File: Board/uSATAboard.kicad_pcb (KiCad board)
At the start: 2 copper layers, 34.5 x 8.4 mm, 8 parts, among them CN2 USATA, P1 CONN_1, P2 CONN_1, P3 CONN_1, P4 CONN_1, P5 CONN_1, P6 CONN_1, P7 CONN_1

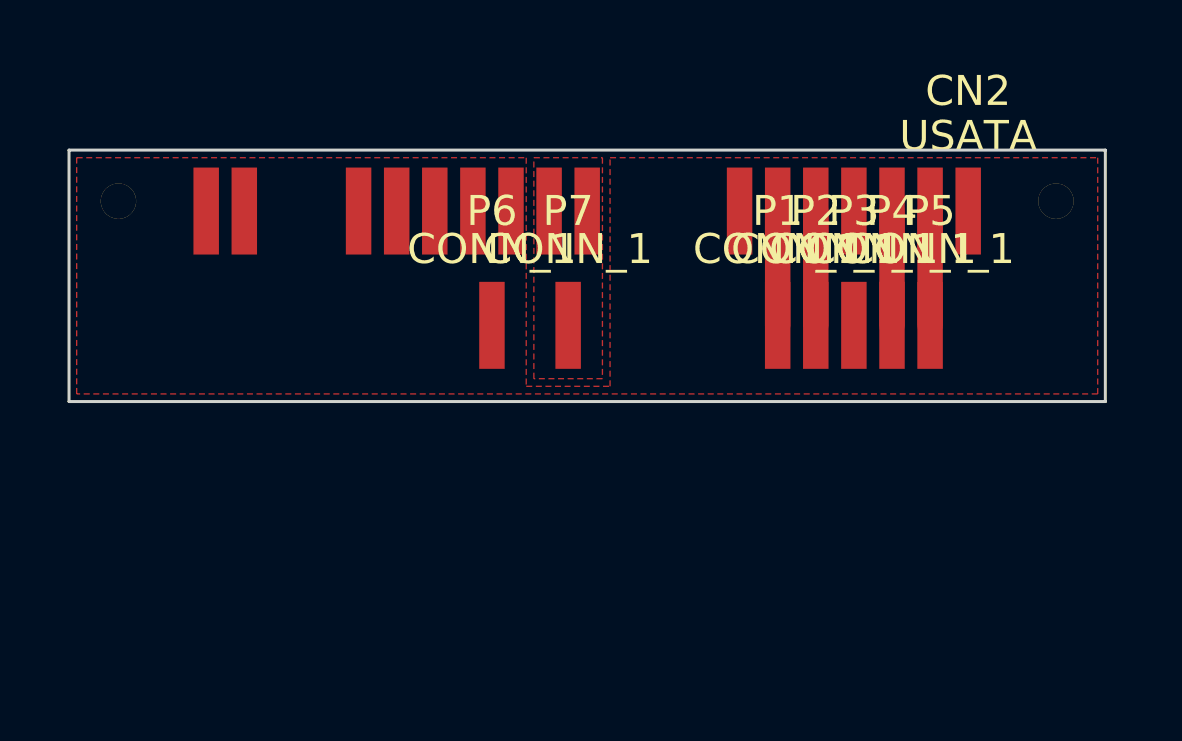
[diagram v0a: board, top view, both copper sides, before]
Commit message: final
for now
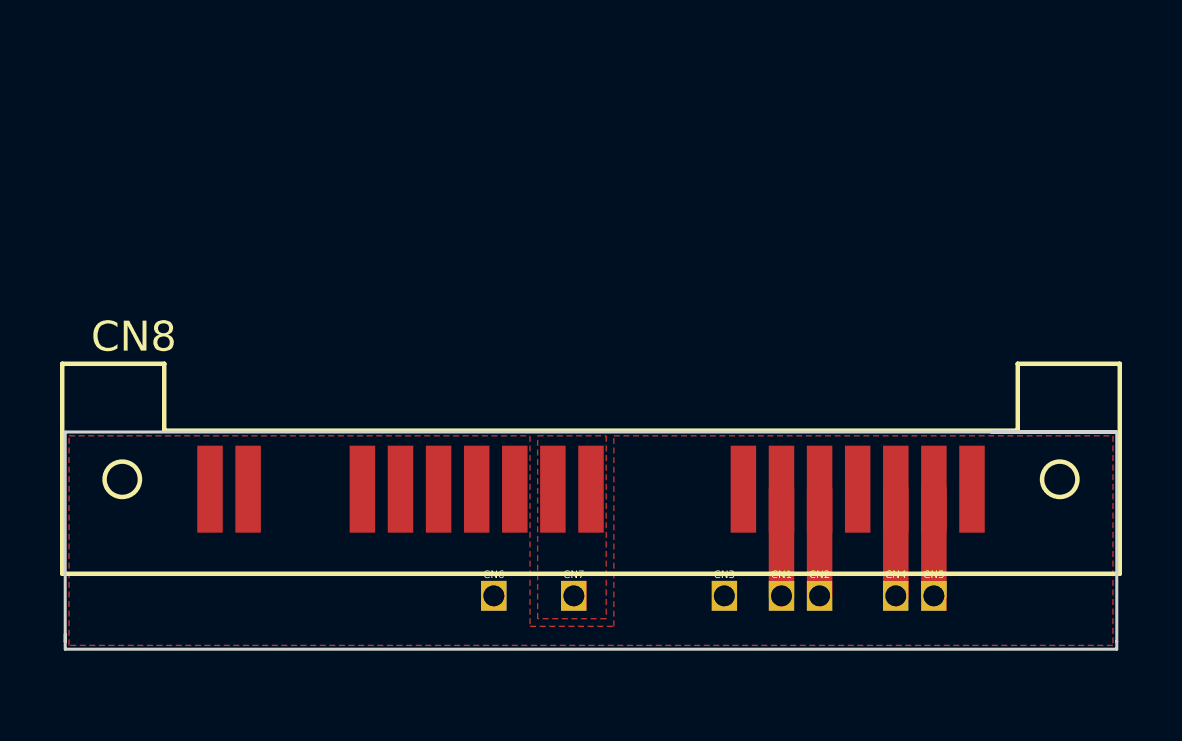
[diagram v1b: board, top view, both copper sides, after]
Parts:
- removed P1, P2, P3, P4, P5, P6, P7: CONN_1, smd_usata
- added CN1: B+, eeepc_ssd:CONN1, F.Cu at (153.8, 92.8)
- added CN3: GND, eeepc_ssd:CONN1, F.Cu at (151.9, 92.8)
- added CN4: A-, eeepc_ssd:CONN1, F.Cu at (157.6, 92.8)
- added CN5: A+, eeepc_ssd:CONN1, F.Cu at (158.9, 92.8)
- added CN6: GND, eeepc_ssd:CONN1, F.Cu at (144.2, 92.8)
- added CN7: +3.3V, eeepc_ssd:CONN1, F.Cu at (146.9, 92.8)
- added CN8: USATA, eeepc_ssd:uSATA, F.Cu at (160.1, 89.3)
- CN2: value USATA -> B-; footprint uSATA -> eeepc_ssd:CONN1
- moved CN2 13.8 mm to (155.1, 92.8)
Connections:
- CN2 pad 1: /GND -> B-
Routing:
- net /B-: track 3.81 -> 0.00 mm
- net /B+: track 3.81 -> 0.00 mm
- net /A-: track 3.81 -> 0.00 mm
- net /A+: track 3.81 -> 0.00 mm
- net B-: track 0.00 -> 3.56 mm
- net B+: track 0.00 -> 3.56 mm
- net A-: track 0.00 -> 3.56 mm
- net A+: track 0.00 -> 3.56 mm
- added copper zone on F.Cu, net +3.3V
- added copper zone on F.Cu, net GND
- removed copper zone on F.Cu, net /+3.3V
- removed copper zone on F.Cu, net /GND
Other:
- board size 34.5 x 8.4 mm -> 35.1 x 7.2 mm
- net class Default: clearance 0.15 -> 0.2; via_dia 0.889 -> 0.6; via_drill 0.635 -> 0.4
- rule trace_clearance: 0.15 -> 0.2
- rule trace_min: 0.254 -> 0.2
- rule via_min_drill: 0.508 -> 0.3
- rule via_min_size: 0.889 -> 0.4

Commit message: do it
done
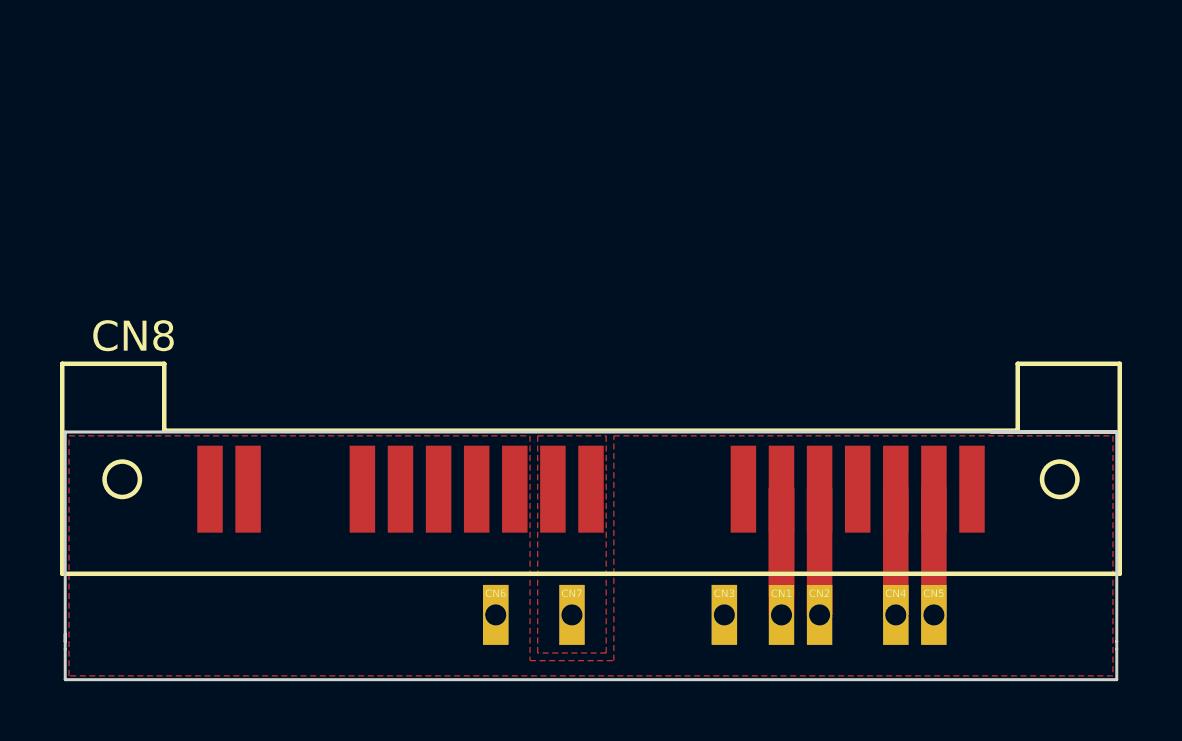
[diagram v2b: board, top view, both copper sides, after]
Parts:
- moved CN6 0.64 mm to (144.3, 93.5)
- moved CN7 0.64 mm to (146.8, 93.5)
- moved CN1 0.63 mm to (153.8, 93.5)
- moved CN2 0.63 mm to (155.1, 93.5)
- moved CN3 0.63 mm to (151.9, 93.5)
- moved CN4 0.63 mm to (157.6, 93.5)
- moved CN5 0.63 mm to (158.9, 93.5)
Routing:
- net B+: track 3.56 -> 7.75 mm
- net B-: track 3.56 -> 4.19 mm
- net A-: track 3.56 -> 4.19 mm
- net A+: track 3.56 -> 4.19 mm
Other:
- board size 35.1 x 7.2 mm -> 35.1 x 8.3 mm
- board text added: "GS"
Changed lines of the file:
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@@
     (links 12)
     (no_connects 0)
-    (area 129.870999 87.325999 165.023001 94.665001)
+    (area 129.546999 83.076 165.347001 95.681001)
     (thickness 1.6)
-    (drawings 8)
-    (tracks 4)
+    (drawings 11)
+    (tracks 5)
     (zones 0)
     (modules 8)
@@
     (mod_text_size 1 1)
     (mod_text_width 0.15)
-    (pad_size 1.5 1.5)
-    (pad_drill 0.6)
+    (pad_size 0.85 2)
+    (pad_drill 0.7)
     (pad_to_mask_clearance 0)
     (aux_axis_origin 0 0)
     (visible_elements 7FFFFFFF)
     (pcbplotparams
-      (layerselection 0x01000_00000001)
+      (layerselection 0x00100_00000000)
       (usegerberextensions false)
-      (excludeedgelayer true)
+      (gerberprecision 5)
+      (excludeedgelayer false)
       (linewidth 0.100000)
       (plotframeref false)
@@
   )
   (module eeepc_ssd:CONN1 (layer F.Cu)
-    (at 153.797 92.837)
+    (at 153.797 93.472)
     (fp_text reference CN1 (at 0 -0.7112) (layer F.SilkS)
       (effects (font (size 0.25 0.25) (thickness 0.0625)))
@@
       (effects (font (size 0.25 0.25) (thickness 0.0625)))
     )
-    (pad 1 thru_hole rect (at 0 0) (size 0.85 1) (drill 0.7) (layers *.Cu *.Mask F.SilkS)
+    (pad 1 thru_hole rect (at 0 0) (size 0.85 2) (drill 0.7) (layers *.Cu *.Mask F.SilkS)
       (net 1 B+))
   )
   (module eeepc_ssd:CONN1 (layer F.Cu)
-    (at 155.067 92.837)
+    (at 155.067 93.472)
     (fp_text reference CN2 (at 0 -0.7112) (layer F.SilkS)
       (effects (font (size 0.25 0.25) (thickness 0.0625)))
@@
       (effects (font (size 0.25 0.25) (thickness 0.0625)))
     )
-    (pad 1 thru_hole rect (at 0 0) (size 0.85 1) (drill 0.7) (layers *.Cu *.Mask F.SilkS)
+    (pad 1 thru_hole rect (at 0 0) (size 0.85 2) (drill 0.7) (layers *.Cu *.Mask F.SilkS)
       (net 2 B-))
   )
   (module eeepc_ssd:CONN1 (layer F.Cu)
-    (at 151.892 92.837)
+    (at 151.892 93.472)
     (fp_text reference CN3 (at 0 -0.7112) (layer F.SilkS)
       (effects (font (size 0.25 0.25) (thickness 0.0625)))
@@
       (effects (font (size 0.25 0.25) (thickness 0.0625)))
     )
-    (pad 1 thru_hole rect (at 0 0) (size 0.85 1) (drill 0.7) (layers *.Cu *.Mask F.SilkS)
-      (net 3 GND))
-  )
-  (module eeepc_ssd:CONN1 (layer F.Cu)
-    (at 157.607 92.837)
+    (pad 1 thru_hole rect (at 0 0) (size 0.85 2) (drill 0.7) (layers *.Cu *.Mask F.SilkS)
+      (net 3 GND))
+  )
+  (module eeepc_ssd:CONN1 (layer F.Cu)
+    (at 157.607 93.472)
     (fp_text reference CN4 (at 0 -0.7112) (layer F.SilkS)
       (effects (font (size 0.25 0.25) (thickness 0.0625)))
@@
       (effects (font (size 0.25 0.25) (thickness 0.0625)))
     )
-    (pad 1 thru_hole rect (at 0 0) (size 0.85 1) (drill 0.7) (layers *.Cu *.Mask F.SilkS)
+    (pad 1 thru_hole rect (at 0 0) (size 0.85 2) (drill 0.7) (layers *.Cu *.Mask F.SilkS)
       (net 4 A-))
   )
   (module eeepc_ssd:CONN1 (layer F.Cu)
-    (at 158.877 92.837)
+    (at 158.877 93.472)
     (fp_text reference CN5 (at 0 -0.7112) (layer F.SilkS)
       (effects (font (size 0.25 0.25) (thickness 0.0625)))
@@
       (effects (font (size 0.25 0.25) (thickness 0.0625)))
     )
-    (pad 1 thru_hole rect (at 0 0) (size 0.85 1) (drill 0.7) (layers *.Cu *.Mask F.SilkS)
+    (pad 1 thru_hole rect (at 0 0) (size 0.85 2) (drill 0.7) (layers *.Cu *.Mask F.SilkS)
       (net 5 A+))
   )
   (module eeepc_ssd:CONN1 (layer F.Cu)
-    (at 144.2085 92.837)
+    (at 144.272 93.472)
     (fp_text reference CN6 (at 0 -0.7112) (layer F.SilkS)
       (effects (font (size 0.25 0.25) (thickness 0.0625)))
@@
       (effects (font (size 0.25 0.25) (thickness 0.0625)))
     )
-    (pad 1 thru_hole rect (at 0 0) (size 0.85 1) (drill 0.7) (layers *.Cu *.Mask F.SilkS)
-      (net 3 GND))
-  )
-  (module eeepc_ssd:CONN1 (layer F.Cu)
-    (at 146.8755 92.837)
+    (pad 1 thru_hole rect (at 0 0) (size 0.85 2) (drill 0.7) (layers *.Cu *.Mask F.SilkS)
+      (net 3 GND))
+  )
+  (module eeepc_ssd:CONN1 (layer F.Cu)
+    (at 146.812 93.472)
     (fp_text reference CN7 (at 0 -0.7112) (layer F.SilkS)
       (effects (font (size 0.25 0.25) (thickness 0.0625)))
@@
       (effects (font (size 0.25 0.25) (thickness 0.0625)))
     )
-    (pad 1 thru_hole rect (at 0 0) (size 0.85 1) (drill 0.7) (layers *.Cu *.Mask F.SilkS)
+    (pad 1 thru_hole rect (at 0 0) (size 0.85 2) (drill 0.7) (layers *.Cu *.Mask F.SilkS)
       (net 6 +3.3V))
   )
@@
       (clearance 0.0001))
   )
+  (gr_line (start 129.921 94.615) (end 129.921 95.631) (angle 90) (layer Edge.Cuts) (width 0.1))
+  (gr_line (start 164.973 94.615) (end 164.973 95.631) (angle 90) (layer Edge.Cuts) (width 0.1))
+  (gr_text GS (at 137.922 92.964) (layer Dwgs.User)
+    (effects (font (size 1 1) (thickness 0.25)))
+  )
   (gr_line (start 164.973 94.361) (end 164.973 94.615) (angle 90) (layer Edge.Cuts) (width 0.1))
   (gr_line (start 129.921 94.361) (end 129.921 94.615) (angle 90) (layer Edge.Cuts) (width 0.1))
@@
   (gr_line (start 129.921 94.107) (end 129.921 94.361) (angle 90) (layer Edge.Cuts) (width 0.1))
   (gr_line (start 129.921 87.376) (end 164.973 87.376) (angle 90) (layer Edge.Cuts) (width 0.1))
-  (gr_line (start 164.973 94.615) (end 129.921 94.615) (angle 90) (layer Edge.Cuts) (width 0.1))
+  (gr_line (start 164.973 95.631) (end 129.921 95.631) (angle 90) (layer Edge.Cuts) (width 0.1))
   (gr_line (start 160.782 87.376) (end 164.973 87.376) (angle 90) (layer Edge.Cuts) (width 0.1))
+  (segment (start 153.797 89.281) (end 153.797 93.472) (width 0.85) (layer F.Cu) (net 1) (status C00000))
   (segment (start 153.797 92.837) (end 153.797 89.281) (width 0.85) (layer F.Cu) (net 1))
-  (segment (start 155.067 92.837) (end 155.067 89.281) (width 0.85) (layer F.Cu) (net 2))
-  (segment (start 157.607 92.837) (end 157.607 89.281) (width 0.85) (layer F.Cu) (net 4))
-  (segment (start 158.877 92.837) (end 158.877 89.281) (width 0.85) (layer F.Cu) (net 5))
+  (segment (start 155.067 93.472) (end 155.067 89.281) (width 0.85) (layer F.Cu) (net 2) (status 10))
+  (segment (start 157.607 93.472) (end 157.607 89.281) (width 0.85) (layer F.Cu) (net 4) (status 10))
+  (segment (start 158.877 93.472) (end 158.877 89.281) (width 0.85) (layer F.Cu) (net 5) (status 10))
   (zone (net 6) (net_name +3.3V) (layer F.Cu) (hatch edge 0.508)
     (connect_pads yes (clearance 0.254))
@@
     (polygon
       (pts
-        (xy 147.955 93.599) (xy 145.669 93.599) (xy 145.669 87.503) (xy 147.955 87.503) (xy 147.955 93.599)
+        (xy 147.955 94.742) (xy 145.669 94.742) (xy 145.669 87.503) (xy 147.955 87.503) (xy 147.955 94.742)
       )
     )
@@
     (polygon
       (pts
-        (xy 145.415 93.853) (xy 148.209 93.853) (xy 148.209 87.503) (xy 164.846 87.503) (xy 164.846 94.488)
-        (xy 130.048 94.488) (xy 130.048 87.503) (xy 145.415 87.503) (xy 145.415 93.853)
+        (xy 145.415 94.996) (xy 148.209 94.996) (xy 148.209 87.503) (xy 164.846 87.503) (xy 164.846 95.504)
+        (xy 130.048 95.504) (xy 130.048 87.503) (xy 145.415 87.503) (xy 145.415 94.996)
       )
     )
